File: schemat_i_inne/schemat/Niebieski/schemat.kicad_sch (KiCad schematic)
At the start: 34 parts, among them J1 Hole1, J2 Hole2, J3 Hole3, J4 Hole4, J5 RJ45, J6 Conn_01x01_Male, J7 Conn_01x01_Male, SW1 SW_DIP_x01, SW2 Left, SW3 Up, SW4 Down, SW5 Right, SW6 Jump, SW7 Punch, U1 ATmega32A-AU, U2 L7805, U3 WG12864B-STBL, U4 LF33_TO252, U5 SN74LS07, U6 SD, Y1 16Mhz

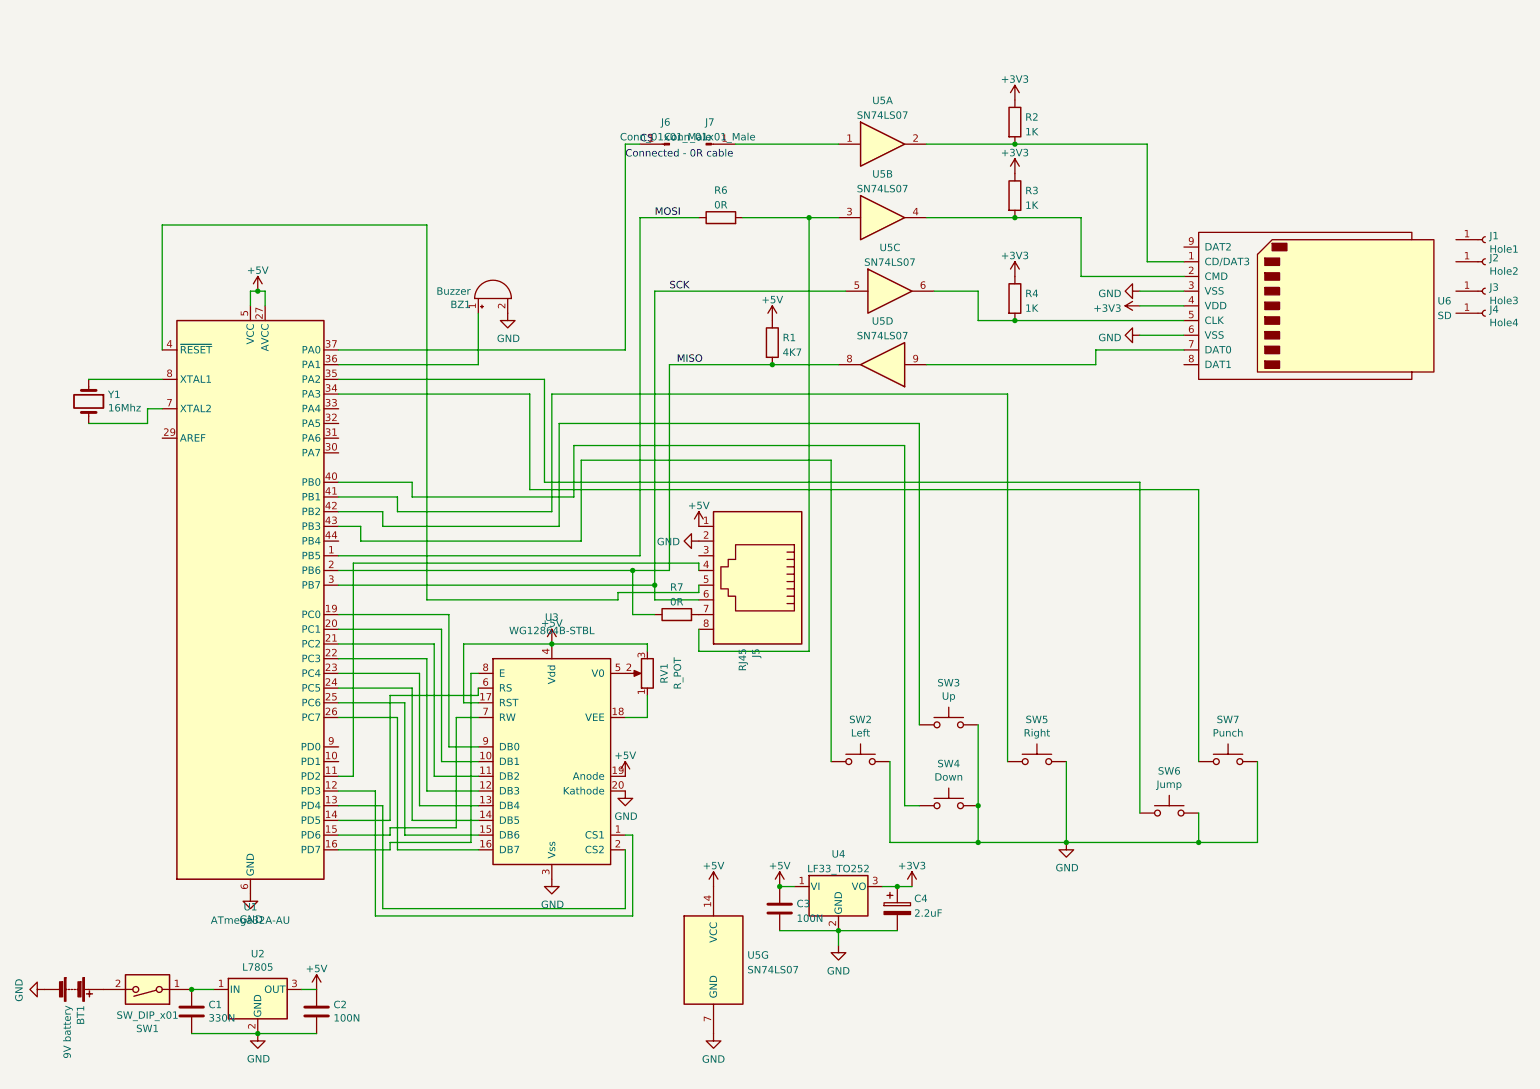
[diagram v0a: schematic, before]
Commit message: new version of schema and board
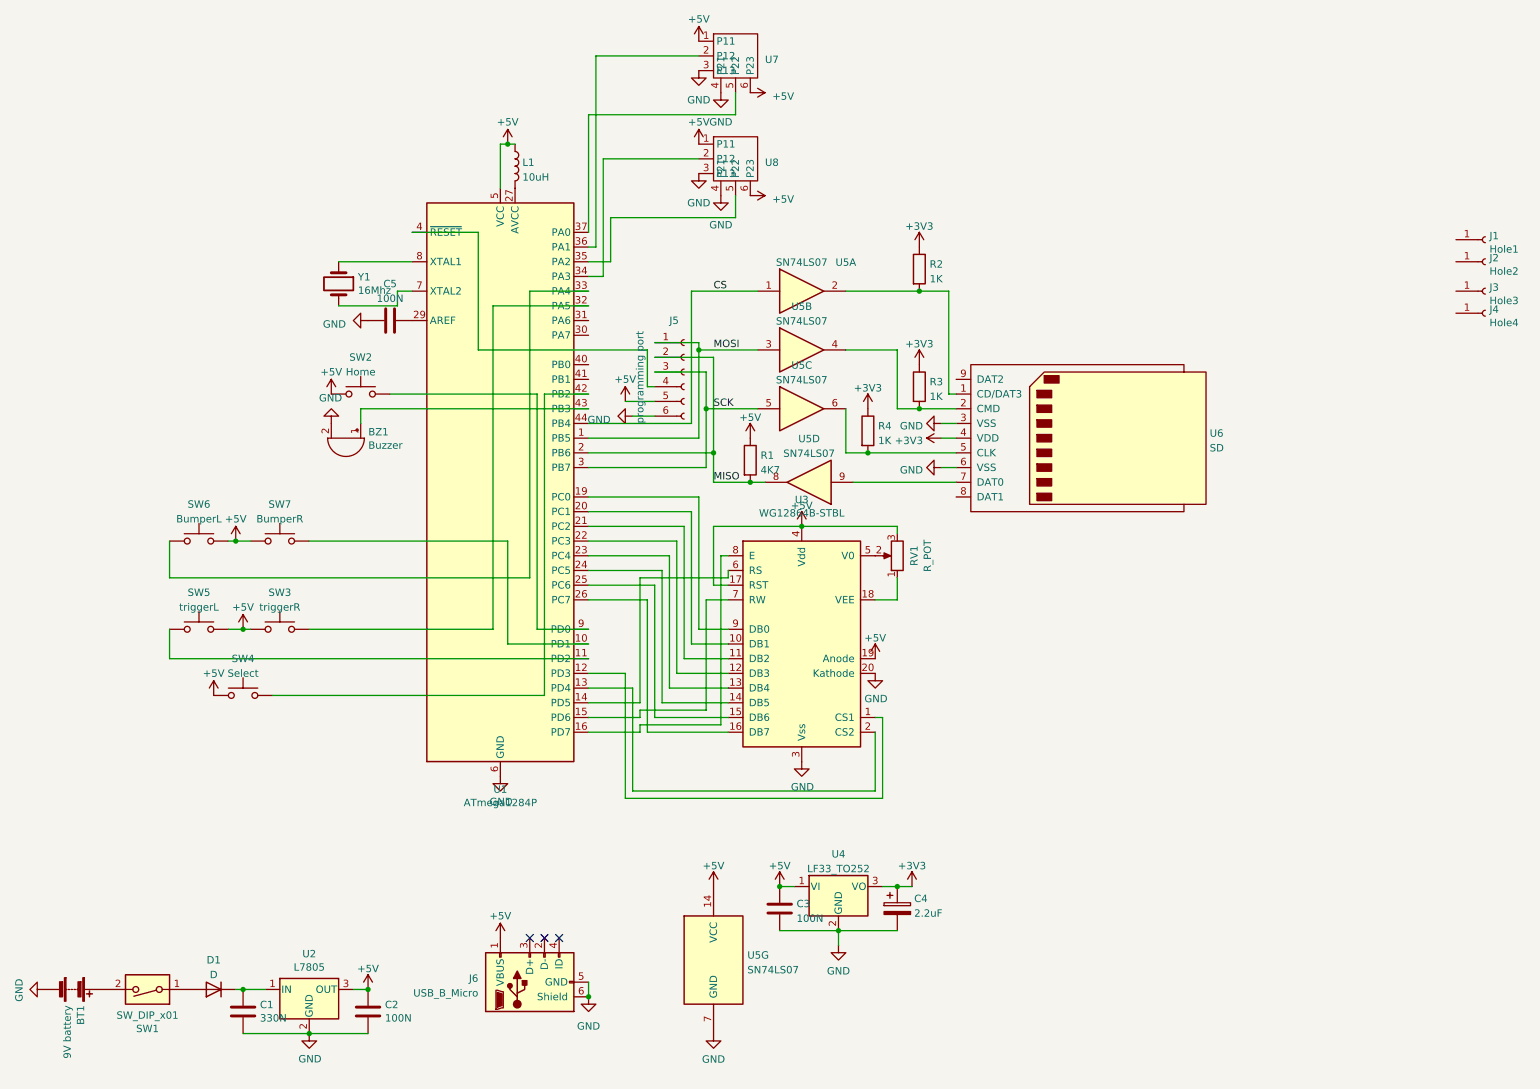
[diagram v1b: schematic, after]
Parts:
- removed J5: RJ45, Connector_RJ:RJ45_Amphenol_54602-x08_Horizontal, symbol Connector:RJ45
- removed J6, J7: Conn_01x01_Male, Connector_PinHeader_2.54mm:PinHeader_1x01_P2.54mm_Vertical, symbol Connector:Conn_01x01_Male
- removed R6: 0R, Resistor_THT:R_Axial_DIN0207_L6.3mm_D2.5mm_P10.16mm_Horizontal, symbol Device:R
- removed R7: 0R, Resistor_THT:R_Axial_DIN0204_L3.6mm_D1.6mm_P2.54mm_Vertical, symbol Device:R
- added C5: 100N, Capacitor_SMD:C_0805_2012Metric, symbol Device:C
- added D1: D, Diode_SMD:D_0201_0603Metric, symbol Device:D
- added J5: programming port, Connector_PinSocket_2.54mm:PinSocket_1x06_P2.54mm_Vertical, symbol Connector:Conn_01x06_Socket
- added J6: USB_B_Micro, Connector_USB:USB_Micro-AB_Molex_47590-0001, symbol Connector:USB_B_Micro
- added L1: 10uH, Inductor_SMD:L_6.3x6.3_H3, symbol Device:L
- added U7, U8: ~, joystick:joystickTHT, symbol joystick:joystickTHT
- BT1: footprint Connector_PinHeader_2.54mm:PinHeader_1x02_P2.54mm_Vertical -> Connector_PinSocket_2.54mm:PinSocket_1x02_P2.54mm_Vertical
- C1, C2, C3: footprint Connector_PinHeader_2.54mm:PinHeader_1x02_P2.54mm_Vertical -> Capacitor_SMD:C_0805_2012Metric
- C4: footprint Connector_PinHeader_2.54mm:PinHeader_1x02_P2.54mm_Vertical -> Capacitor_SMD:CP_Elec_6.3x5.4_Nichicon
- SW1: footprint Connector_PinHeader_2.54mm:PinHeader_1x03_P2.54mm_Vertical -> Button_Switch_SMD:SW_DIP_SPSTx01_Slide_Copal_CVS-01xB_W5.9mm_P1mm
- SW2: value Left -> Home; footprint Button_Switch_THT:SW_PUSH-12mm -> Button_Switch_SMD:SW_Push_1P1T_NO_6x6mm_H9.5mm
- SW3: value Up -> triggerR; footprint Button_Switch_THT:SW_PUSH-12mm -> Button_Switch_THT:SW_Tactile_SPST_Angled_PTS645Vx31-2LFS
- SW4: value Down -> Select; footprint Button_Switch_THT:SW_PUSH-12mm -> Button_Switch_SMD:SW_Push_1P1T_NO_6x6mm_H9.5mm
- SW5: value Right -> triggerL; footprint Button_Switch_THT:SW_PUSH-12mm -> Button_Switch_THT:SW_Tactile_SPST_Angled_PTS645Vx31-2LFS
- SW6: value Jump -> BumperL; footprint Button_Switch_THT:SW_PUSH-12mm -> Button_Switch_THT:SW_Tactile_SPST_Angled_PTS645Vx31-2LFS
- SW7: value Punch -> BumperR; footprint Button_Switch_THT:SW_PUSH-12mm -> Button_Switch_THT:SW_Tactile_SPST_Angled_PTS645Vx31-2LFS
- U1: value ATmega32A-AU -> ATmega1284P
- U2: footprint Package_TO_SOT_THT:TO-220-3_Vertical -> Package_TO_SOT_SMD:TO-252-2
- U5: footprint Package_DIP:DIP-14_W7.62mm_LongPads -> Package_SO:SO-14_3.9x8.65mm_P1.27mm
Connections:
- net SCK is gone; now on net MISO: U1.3 (PB7), U5.5
- net +5V: now also SW2.1, SW3.1, SW4.1, SW5.2, SW6.2, SW7.1, J5.5 (Pin_5), J6.1 (VBUS), L1.1, U7.1 (P11), U7.6 (P23), U8.1 (P11), U8.6 (P23); no longer U1.27 (AVCC)
- net CS: now also U1.44 (PB4), U5.1; no longer U1.37 (PA0)
- net GND: now also C5.2, J5.6 (Pin_6), J6.5 (GND), J6.6 (Shield), U7.3 (P13), U7.4 (P21), U8.3 (P13), U8.4 (P21); no longer SW2.2, SW3.2, SW4.2, SW5.2, SW6.2, SW7.2
- net MISO: now also J5.2 (Pin_2), J5.3 (Pin_3)
- net MOSI: now also U5.3, J5.1 (Pin_1)
- net at U1.42 (PB2): now also SW4.2; no longer SW3.1
- net at U1.40 (PB0): no longer SW4.1
- net at SW5.1: now also U1.11 (PD2); no longer U1.41 (PB1)
- net at U1.43 (PB3): now also BZ1.1 (-); no longer SW2.1
- net at SW6.1: now also U1.33 (PA4); no longer U1.35 (PA2)
- net at U1.34 (PA3): now also U8.2 (P12); no longer SW7.1
- net at U1.10 (PD1): now also SW7.2
- net at U1.29 (AREF): now also C5.1
- net at U1.32 (PA5): now also SW3.2
- net at U1.36 (PA1): now also U7.2 (P12); no longer BZ1.1 (-)
- net at U1.4 (~{RESET}): now also J5.4 (Pin_4)
- net at U1.9 (PD0): now also SW2.2
- net at C1.1, U2.1 (IN): now also D1.1 (K); no longer SW1.1
- new net: L1.2, U1.27 (AVCC)
- new net: U1.35 (PA2), U8.5 (P22)
- new net: U1.37 (PA0), U7.5 (P22)
- new net: D1.2 (A), SW1.1
- no-connect marks 0 -> 3
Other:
- note removed: "Connected - 0R cable"
- moved on the sheet: BZ1, C1, C2, R1, R2, R3, R4, RV1, U1, U2, U3, U5A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
